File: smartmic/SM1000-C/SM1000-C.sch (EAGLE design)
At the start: 188 parts, among them CN1 HDR100-3, CN10 MJ-3523-SMT, CN11 HDR100-3, CN12 HRS-DF11-16DS, CN2 MOLEX-MINI-B-SMT, CN3 RASM722PX, CN4 RJ-45, CN5 MJ-3523-SMT, CN6 SJ-3524-SMT, CN7 MJ-3523-SMT, CN8 SJ-3524-SMT, CN9 MJ-3523-SMT, J1 JMP-2PIN, J3 JMP-2PIN, J4 JMP-2PIN, P1 TPAD50, P10 TPAD50, P11 TPAD50, P12 TPAD50, P13 TPAD50, P14 TPAD50, P15 TPAD50, P16 TPAD50, P17 TPAD50, P18 TPAD50, P19 TPAD50, P2 TPAD50, P20 TPAD50, P21 PAD070-035, P22 PAD070-035, P23 PAD070-035, P24 PAD070-035, P3 TPAD50, P4 TPAD50, P5 TPAD50, P6 TPAD50, P7 TPAD50, P8 TPAD50, P9 TPAD50, SW1 SW-BOURNS-7914S, SW2 SW-BOURNS-7914S, SW3 DPDT, SW4 SW-BOURNS-7914S, SW5 SW-BOURNS-7914J, T1 SM-LP-5001, T2 SM-LP-5001, U1 STM32F405, U2 LD3985M33R, U3 STMPS2141, U4 EMIF02-USB03F2, U5 TPS54329E, U6 LMV341, U7 LMV341, U8 LM386M-1, U9 LMV341

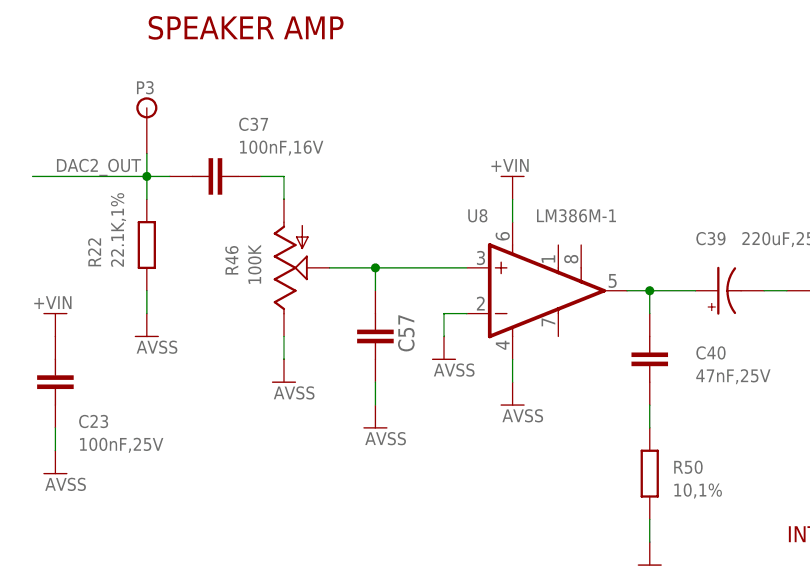
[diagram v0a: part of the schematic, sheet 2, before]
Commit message: Update file & add DIM PDFs  RGB 09/27/14
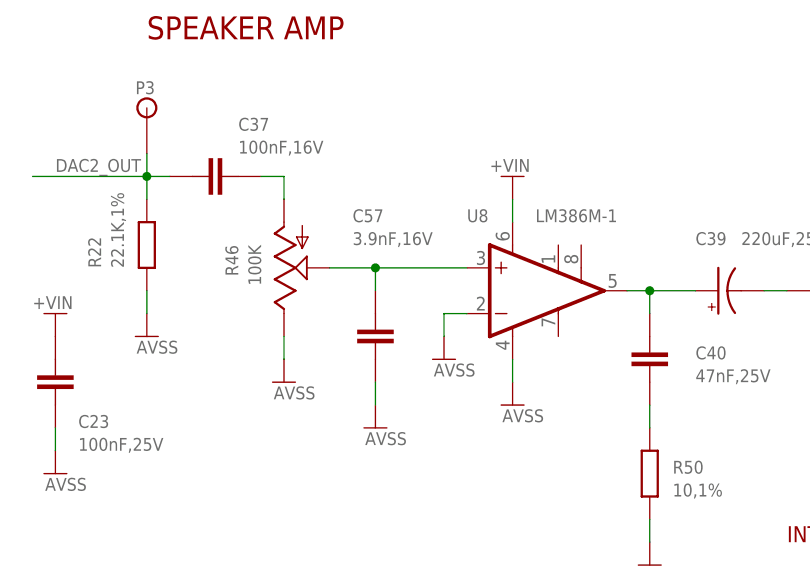
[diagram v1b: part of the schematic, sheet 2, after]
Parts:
- C57: value (none) -> 3.9nF,16V
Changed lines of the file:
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@@
 <part name="R9" library="AA-ipc-7351-resistor" deviceset="RESISTOR_" device="0603" value="1.5K,1%"/>
 <part name="R29" library="AA-ipc-7351-resistor" deviceset="RESISTOR_" device="0603" value="1.5K,1%"/>
-<part name="C57" library="AA-ipc-7351-capacitor" deviceset="CAPACITOR_" device="0603"/>
+<part name="C57" library="AA-ipc-7351-capacitor" deviceset="CAPACITOR_" device="0603" value="3.9nF,16V"/>
 <part name="U$50" library="A-SUPPLY2" deviceset="AVSS" device=""/>
 <part name="CN12" library="SM1000" deviceset="HRS-DF11-16DS" device=""/>
@@
 <attribute name="VALUE" x="132.08" y="132.08" size="1.4224" layer="96" ratio="9"/>
 </instance>
-<instance part="C57" gate="G$1" x="45.72" y="50.8" rot="R270"/>
+<instance part="C57" gate="G$1" x="45.72" y="50.8" smashed="yes" rot="R270">
+<attribute name="NAME" x="43.18" y="63.5" size="1.4224" layer="95"/>
+<attribute name="VALUE" x="43.18" y="60.96" size="1.4224" layer="96"/>
+</instance>
 <instance part="U$50" gate="G$1" x="45.72" y="43.18"/>
 <instance part="CN12" gate="G$1" x="279.4" y="172.72"/>
